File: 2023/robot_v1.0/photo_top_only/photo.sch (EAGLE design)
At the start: 22 parts

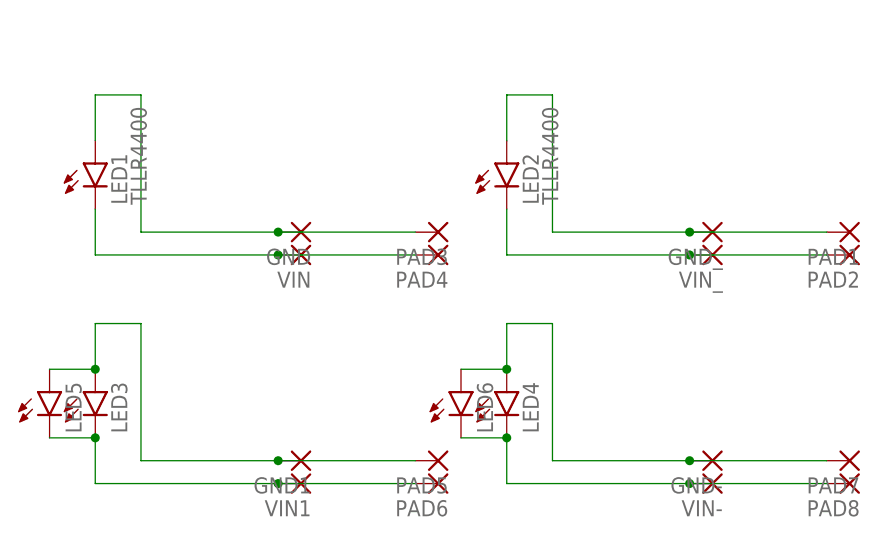
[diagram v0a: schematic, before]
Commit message: some fix
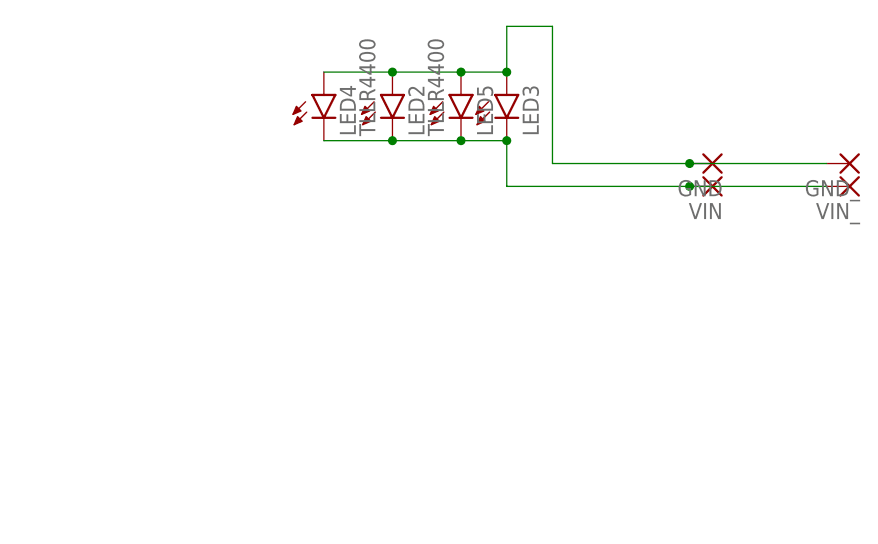
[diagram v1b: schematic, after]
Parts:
- removed GND-, GND1, PAD1, PAD2, PAD3, PAD4, PAD5, PAD6, PAD7, PAD8, VIN-, VIN1: (no value), wirepad:SMD2
- removed LED1: TLLR4400, led:TLLR4400
- removed LED6: (no value), led:LEDCHIP-LED0805
- LED4: value (none) -> TLLR4400; device led:LEDCHIP-LED0805 -> led:TLLR4400
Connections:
- removed net N$1: LED1.C, PAD4.P, VIN.P
- removed net N$2: GND.P, LED1.A, PAD3.P
- removed net N$4: LED2.C, PAD2.P, VIN_.P
- removed net N$6: LED3.C, LED5.C, PAD6.P, VIN1.P
- removed net N$7: GND-.P, LED4.A, LED6.A, PAD7.P
- removed net N$8: LED4.C, LED6.C, PAD8.P, VIN-.P
- net N$3: now also LED2.C, LED3.C, LED4.C, LED5.C, VIN.P, VIN_.P; no longer GND_.P, LED2.A, PAD1.P
- net N$5: now also GND.P, GND_.P, LED2.A, LED4.A; no longer GND1.P, PAD5.P
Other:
- moved on the sheet: GND, GND_, LED2, LED3, LED4, LED5, VIN, VIN_
